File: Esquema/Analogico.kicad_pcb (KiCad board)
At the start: 2 copper layers, 56.7 x 81.8 mm, 43 parts, among them J1 Conex_bat, J2 Panel Solar, J3 Galga_1, J4 Galga_2, P1 USB_C_Plug_USB2.0, U1 REF3020AIDBZT, U10 NUCLEO-F429ZI, U2 INA826AIDR, U3 TP4057, U4 INA826AIDR, U5 INA826AIDR, U6 XL006, U7 TLV75733PDBV, U8 TLV75733PDBV

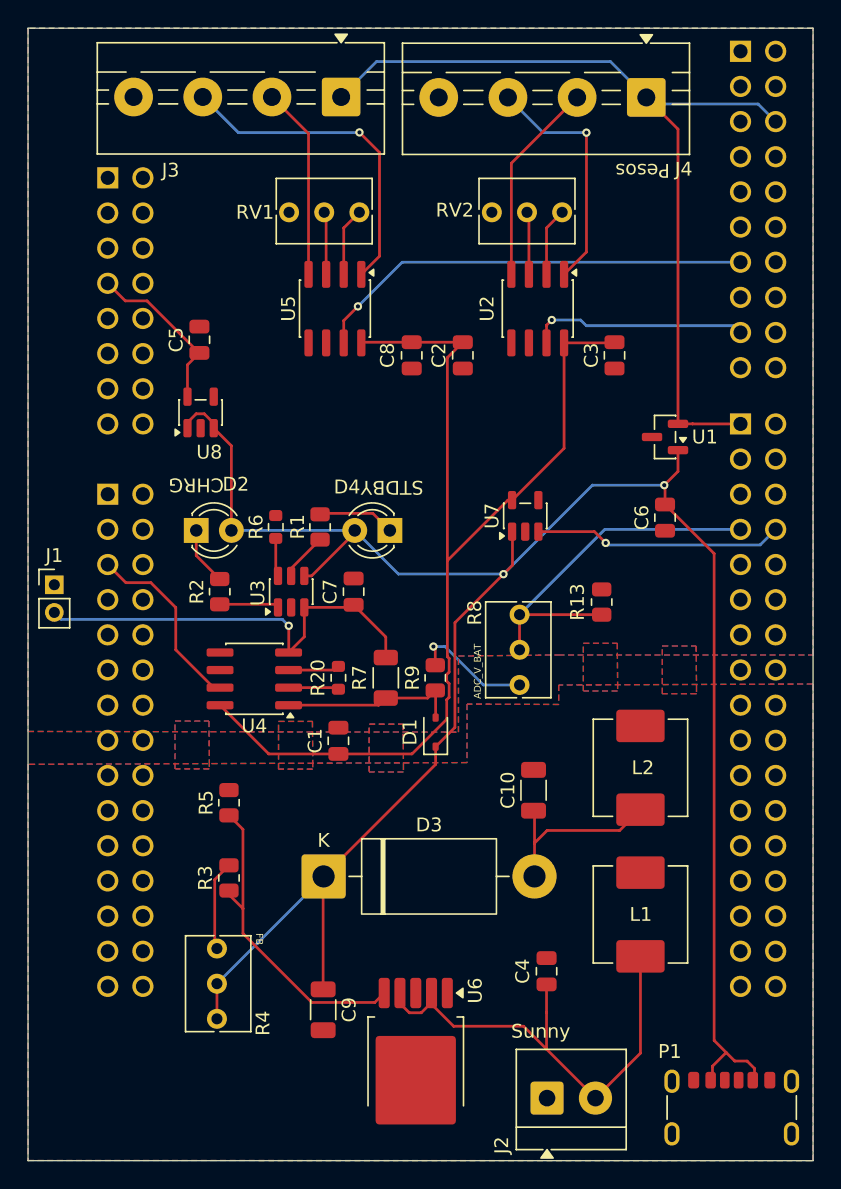
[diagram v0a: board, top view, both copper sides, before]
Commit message: Cambios en el principal y en el adc
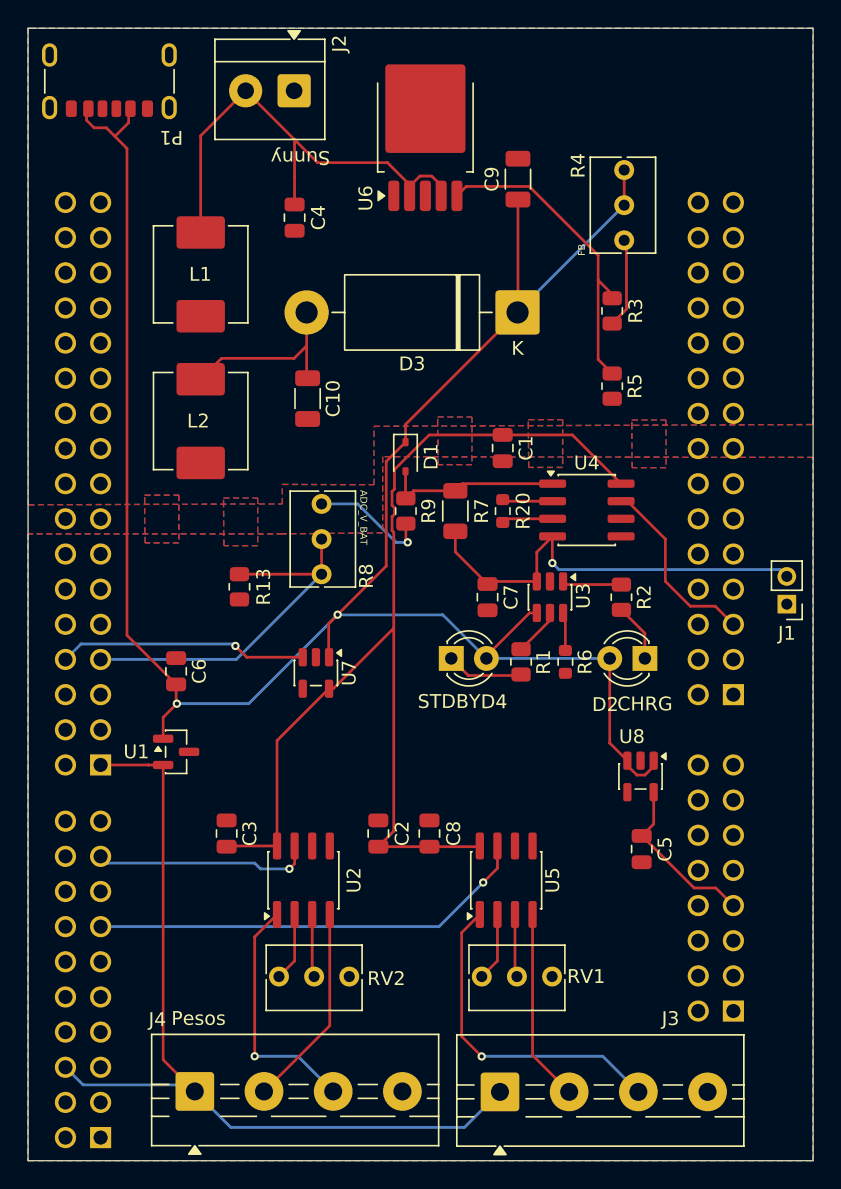
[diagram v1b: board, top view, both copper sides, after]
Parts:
- moved P1 88.6 mm to (90.9, 49.5), turned to 180 degrees
- moved J4 78.9 mm to (97.0, 123.6), turned to 0 degrees
- moved J2 75.0 mm to (104.2, 51.3), turned to 180 degrees
- moved J3 72.8 mm to (119.1, 123.6), turned to 0 degrees
- moved U6 67.7 mm to (113.7, 53.8), turned to 90 degrees
- moved C9 61.6 mm to (120.4, 57.7), turned to 90 degrees
- moved R4 59.0 mm to (128.1, 62.1), turned to -90 degrees
- moved RV1 58.4 mm to (122.9, 115.3), turned to 0 degrees
- moved C4 57.4 mm to (104.3, 60.5), turned to -90 degrees
- moved RV2 56.2 mm to (108.2, 115.3), turned to 0 degrees
- moved L1 56.1 mm to (97.5, 64.5), turned to -90 degrees
- moved J1 52.9 mm to (139.8, 88.4), turned to 180 degrees
- moved R3 49.4 mm to (127.2, 67.2), turned to 90 degrees
- moved C5 48.7 mm to (129.3, 106.1), turned to -90 degrees
- moved U2 44.6 mm to (104.9, 108.3), turned to 90 degrees
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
